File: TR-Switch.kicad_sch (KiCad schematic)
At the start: 8 parts, among them J1 Conn_Coaxial, J2 Conn_Coaxial, J3 Conn_Coaxial, J4 USB_A, K1 HF3-03

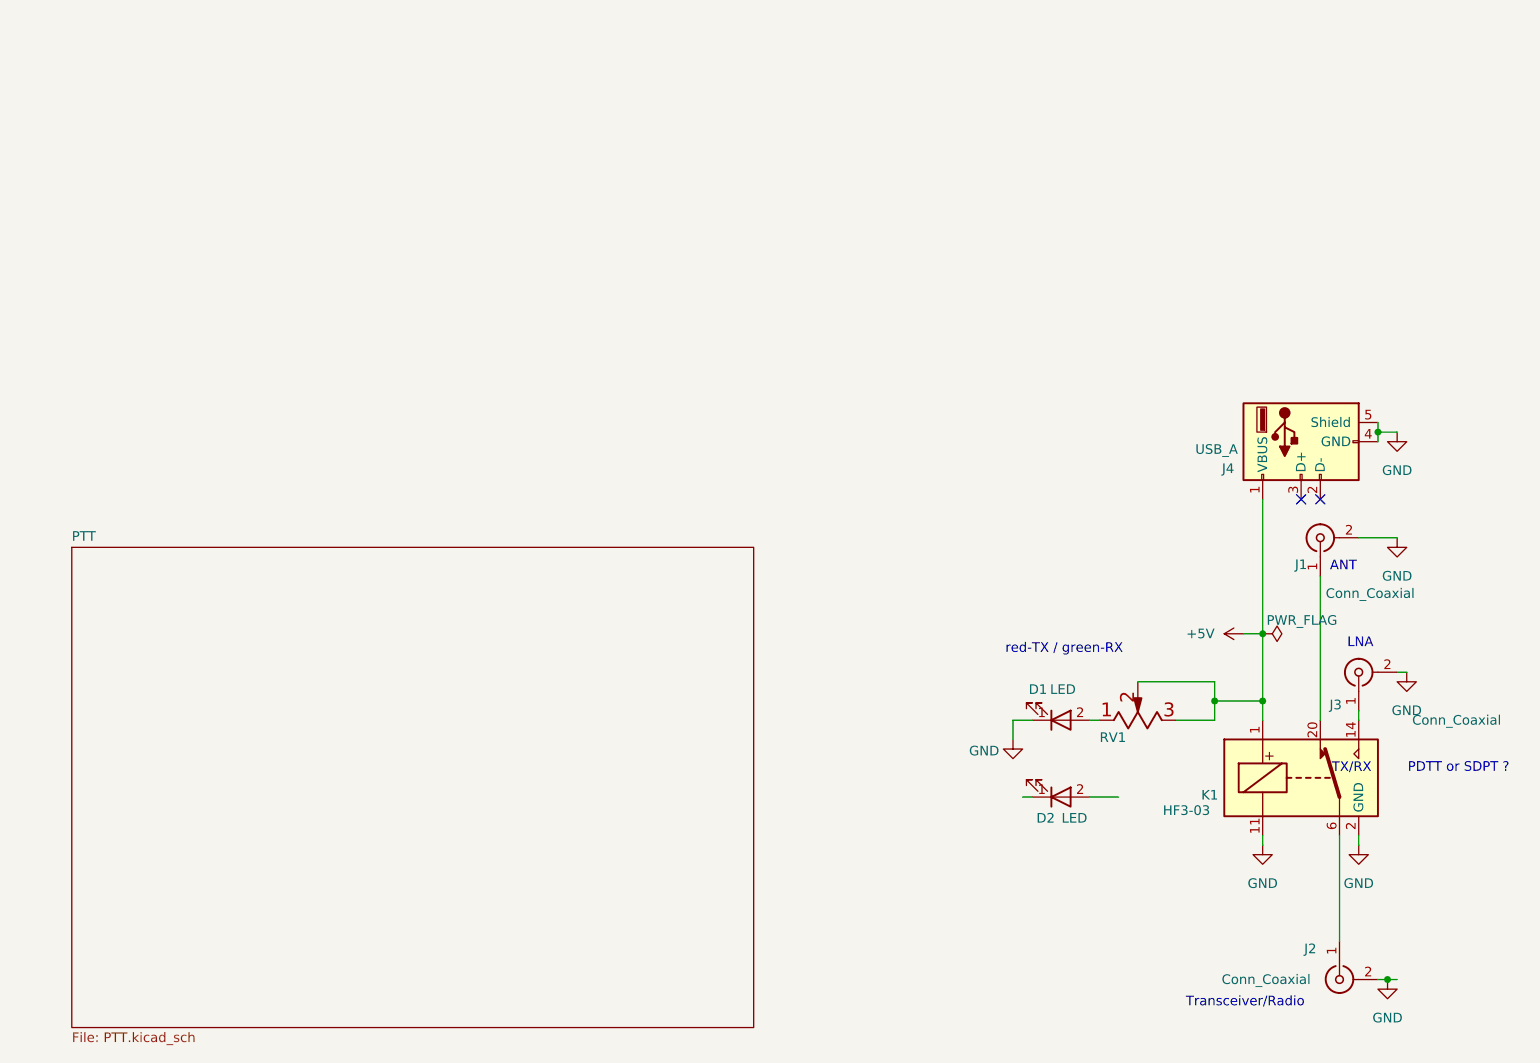
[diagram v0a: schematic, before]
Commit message: -docu + comments -new layout
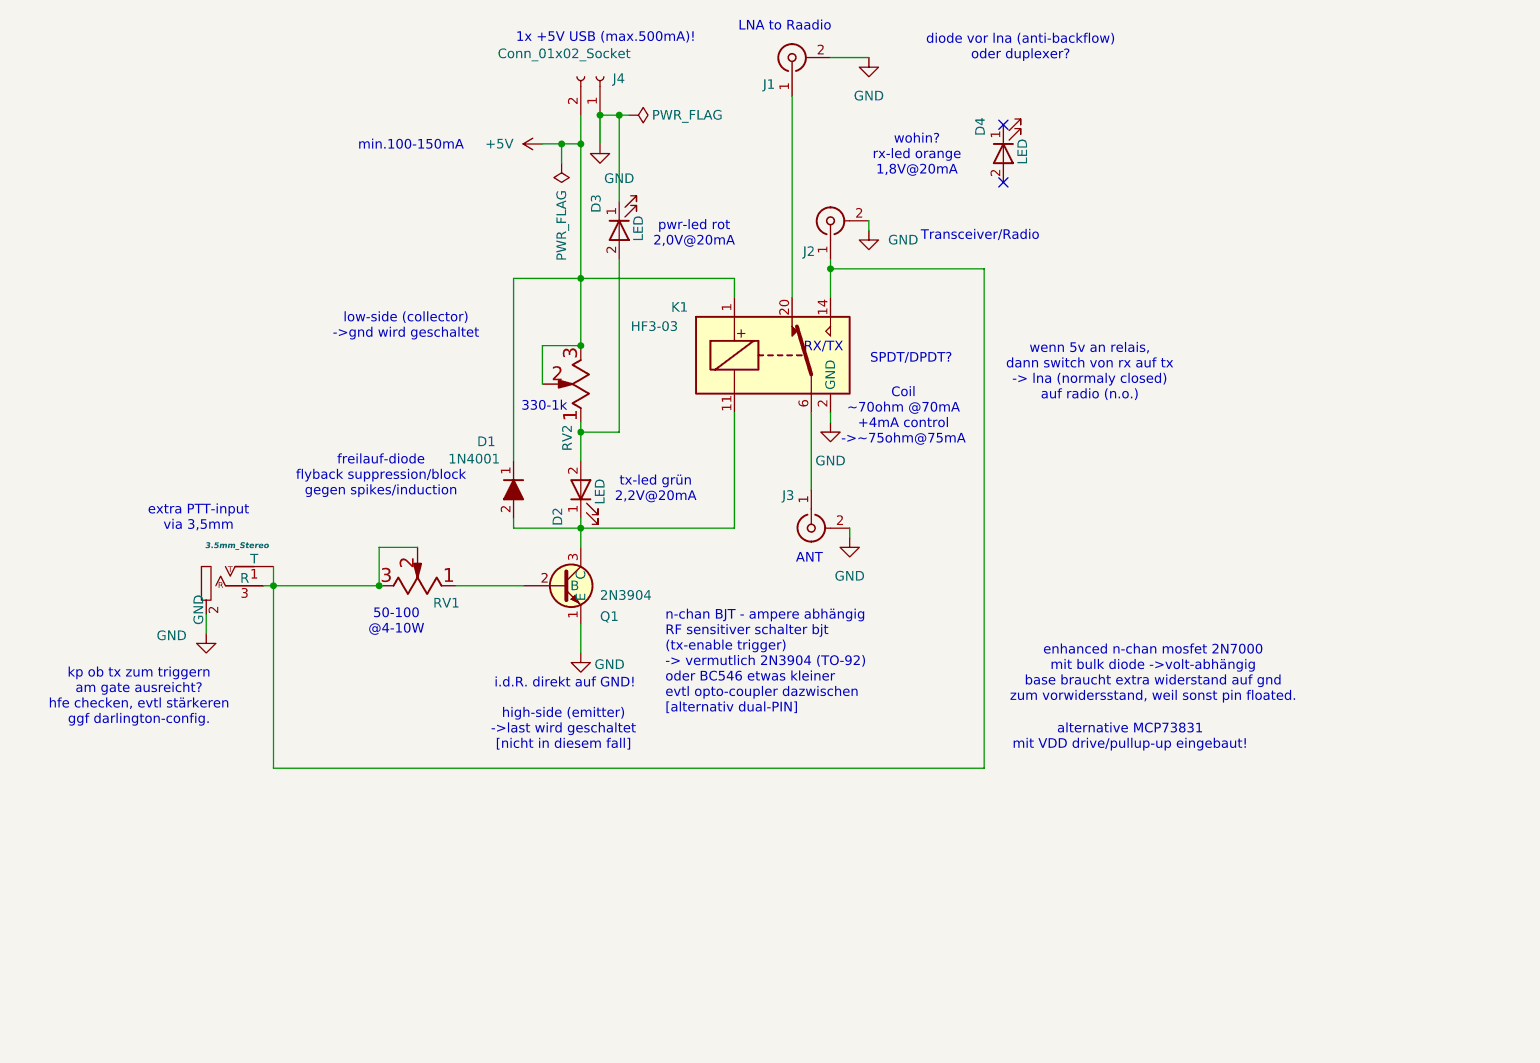
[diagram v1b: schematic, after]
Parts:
- removed D1: LED, LED_THT:LED_D5.0mm, symbol Device:LED
- removed J4: USB_A, Connector_USB:USB_A_Receptacle_GCT_USB1046, symbol Connector:USB_A
- added D1: 1N4001, PCM_Diode_THT_AKL:D_DO-41_SOD81_P7.62mm_Horizontal, symbol PCM_Diode_AKL:1N4001
- added D3, D4: LED, LED_THT:LED_D5.0mm, symbol Device:LED
- added J4: Conn_01x02_Socket, Connector_PinSocket_2.54mm:PinSocket_1x02_P2.54mm_Vertical, symbol Connector:Conn_01x02_Socket
- added J5: 3.5mm_Stereo_SymSmall_0.05, KSJ:Jack_3.5mm_CUI_SJ1-3533NG_Horizontal-wodo, symbol PCM_4ms_Jack:3.5mm_Stereo_SymSmall_0.05
- added Q1: 2N3904, PCM_Package_TO_SOT_THT_AKL:TO-92_Inline_Wide_EBC, symbol PCM_Transistor_BJT_AKL:2N3904
- added RV2: 1kOhm, Potentiometer_THT:Potentiometer_Bourns_3386C_Horizontal, symbol PCM_Generic:R-potentiometer,IEEE,symmetric
- J3: footprint Connector_Coaxial:SMA_Amphenol_132289_EdgeMount -> Connector_Coaxial:BNC_TEConnectivity_1478035_Horizontal
- RV1: value 10kOhm -> 50Ohm
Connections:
- net +5V: now also D1.1 (K), J4.2 (Pin_2), RV2.2 (b), RV2.3 (c); no longer RV1.2 (b), RV1.3 (c)
- net GND: now also D3.1 (K), J4.1 (Pin_1), J5.2 (GND), Q1.1 (E); no longer K1.11
- net at RV1.1 (a): now also Q1.2 (B)
- net at K1.14: now also J2.1 (In), RV1.2 (b), RV1.3 (c), J5.1 (T), J5.3 (R); no longer J3.1 (In)
- net at K1.6: now also J3.1 (In); no longer J2.1 (In)
- net at D2.1 (K): now also K1.11, D1.2 (A), Q1.3 (C)
- net at D2.2 (A): now also D3.2 (A), RV2.1 (a)
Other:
- removed sheet PTT
- note added: "1x +5V USB (max.500mA)!"
- note added: "330-1k"
- note added: "50-100 @4-10W"
- note added: "Coil ~70ohm @70mA +4mA control ->~75ohm@75mA"
- note added: "LNA to Raadio"
- note added: "RX/TX"
- note added: "SPDT/DPDT?"
- note added: "alternative MCP73831 mit VDD drive/pullup-up eingebaut!"
- note added: "diode vor lna (anti-backflow) oder duplexer?"
- note added: "enhanced n-chan mosfet 2N7000 mit bulk diode ->volt-abhängig base braucht extra widerstand auf gnd zum vorwidersstand, weil sonst pin floated."
- note added: "extra PTT-input via 3,5mm"
- note added: "freilauf-diode flyback suppression/block gegen spikes/induction"
- note added: "high-side (emitter) ->last wird geschaltet [nicht in diesem fall]"
- note added: "i.d.R. direkt auf GND!"
- note added: "kp ob tx zum triggern am gate ausreicht? hfe checken, evtl stärkeren ggf darlington-config."
- note added: "low-side (collector) ->gnd wird geschaltet"
- note added: "min.100-150mA"
- note added: "n-chan BJT - ampere abhängig RF sensitiver schalter bjt (tx-enable trigger) -> vermutlich 2N3904 (TO-92) oder BC546 etwas kleiner evtl opto-coupler dazwischen [alternativ dual-PIN]"
- note added: "pwr-led rot 2,0V@20mA"
- note added: "tx-led grün 2,2V@20mA"
- note added: "wenn 5v an relais, dann switch von rx auf tx -> lna (normaly closed) auf radio (n.o.)"
- note added: "wohin? rx-led orange 1,8V@20mA"
- note removed: "LNA"
- note removed: "PDTT or SDPT ?"
- note removed: "TX/RX"
- note removed: "red-TX / green-RX"
- moved on the sheet: J1, K1
